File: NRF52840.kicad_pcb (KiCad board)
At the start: 2 copper layers, 31.2 x 11.3 mm, 26 parts, among them J1 Conn_01x04, J2 USB_A, U1 nRF52840, Y1 32M

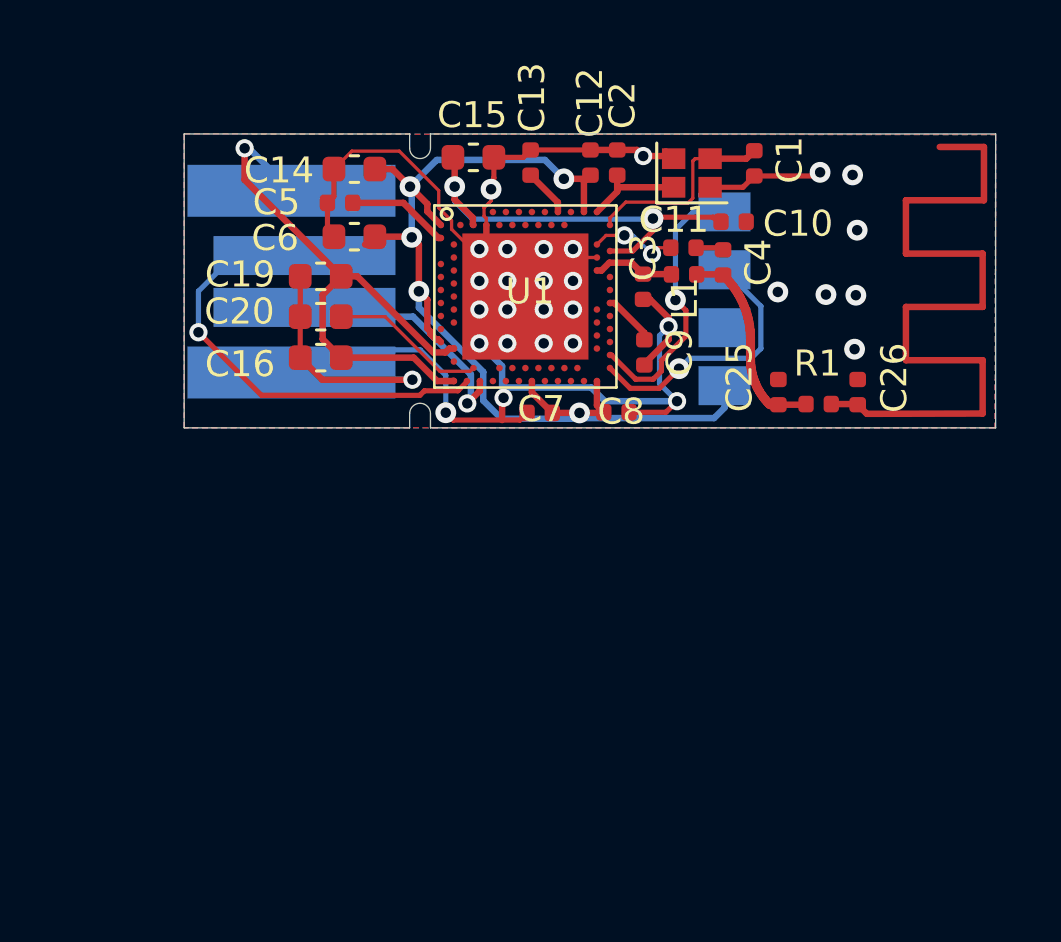
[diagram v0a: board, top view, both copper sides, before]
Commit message: ...
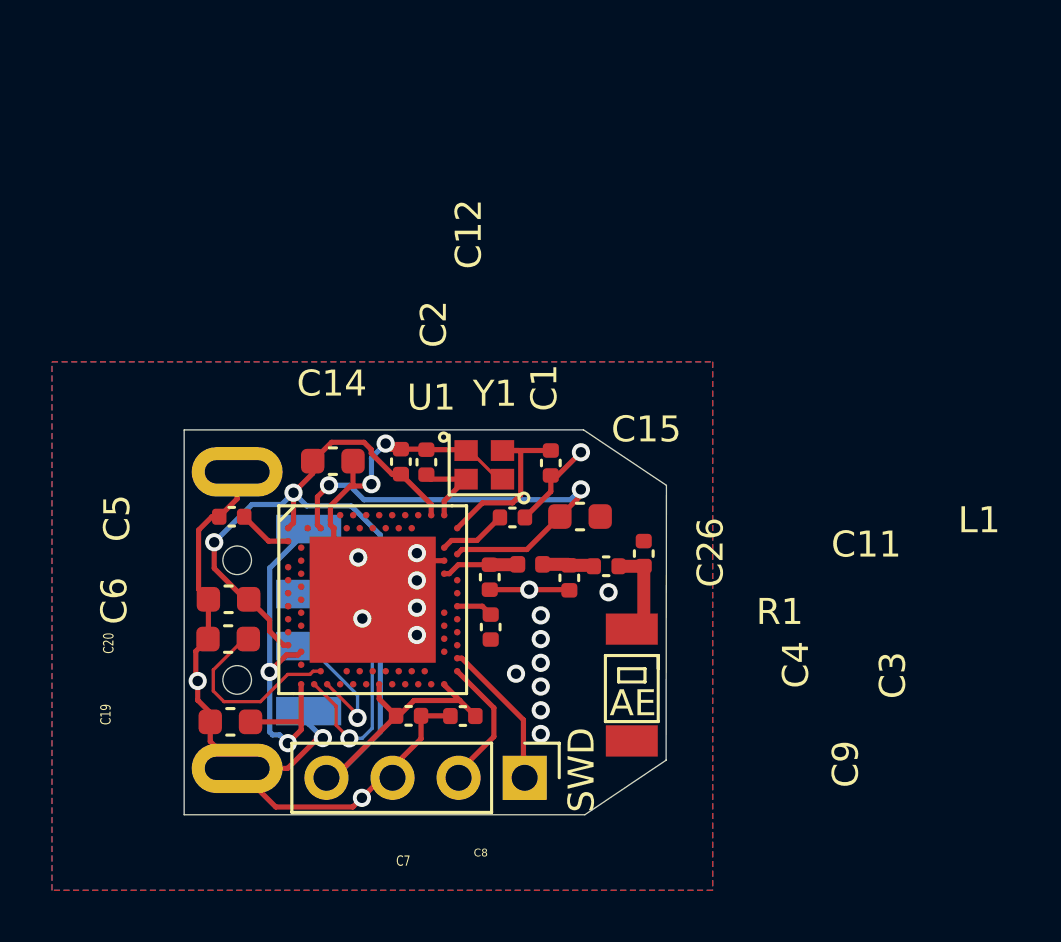
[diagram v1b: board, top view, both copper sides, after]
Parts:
- removed C10, C13, C25: NC, Capacitor_SMD:C_0402_1005Metric
- removed C16: 4.7uF, Capacitor_SMD:C_0603_1608Metric
- removed J1: Conn_01x04, zhangxiaofei:SWD
- added AE: Antenna, zhangxiaofei:2.4g_ANTENNA, F.Cu at (107.2, 141.8)
- added SWD: Conn_01x04, Connector_PinHeader_2.54mm:PinHeader_1x04_P2.54mm_Vertical, F.Cu at (103.1, 145.5)
- J2: footprint zhangxiaofei:USB_PCB -> Connector_USB:USB_A_CNCTech_1001-011-01101_Horizontal
- U1: footprint Package_DFN_QFN:Nordic_AQFN-73-1EP_7x7mm_P0.5mm -> zhangxiaofei:Nordic_AQFN-73-1EP_7x7mm_P0.5mm
- moved C19 17.5 mm to (91.8, 143.3)
- moved J2 15.9 mm to (85.2, 139.4), turned to 180 degrees
- moved C6 14.8 mm to (91.7, 138.6)
- moved C15 14.4 mm to (105.2, 135.4)
- moved C1 13.9 mm to (104.1, 133.3)
- moved Y1 13.8 mm to (101.6, 133.4)
- moved C2 13.7 mm to (99.3, 133.3)
- moved C12 13.6 mm to (98.4, 133.3)
- moved C4 13.5 mm to (104.8, 137.8), turned to 270 degrees
- moved C8 13.1 mm to (100.7, 143.1), turned to 180 degrees
- moved U1 13.1 mm to (97.3, 138.6)
- moved C20 12.9 mm to (91.7, 140.1)
- moved C5 12.8 mm to (91.9, 135.4)
- moved C7 12.7 mm to (98.7, 143.1), turned to 0 degrees
- moved C3 12.6 mm to (101.8, 137.7)
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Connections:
- U1 pad A10: Net-(U1-PadA10) -> (no net)
- U1 pad A12: Net-(U1-PadA12) -> (no net)
- U1 pad A14: Net-(U1-PadA14) -> (no net)
- U1 pad A16: Net-(U1-PadA16) -> (no net)
- U1 pad A18: Net-(C13-Pad2) -> (no net)
- U1 pad A20: Net-(U1-PadA20) -> (no net)
- U1 pad A8: Net-(U1-PadA8) -> (no net)
- U1 pad AB2: Net-(U1-PadAB2) -> (no net)
- U1 pad AC11: Net-(U1-PadAC11) -> (no net)
- U1 pad AC13: Net-(U1-PadAC13) -> (no net)
- U1 pad AC15: Net-(U1-PadAC15) -> (no net)
- U1 pad AC17: Net-(U1-PadAC17) -> (no net)
- U1 pad AC19: Net-(U1-PadAC19) -> (no net)
- U1 pad AC21: Net-(U1-PadAC21) -> (no net)
- U1 pad AC9: Net-(U1-PadAC9) -> (no net)
- U1 pad AD10: Net-(U1-PadAD10) -> (no net)
- U1 pad AD12: Net-(U1-PadAD12) -> (no net)
- U1 pad AD16: Net-(U1-PadAD16) -> (no net)
- U1 pad AD18: Net-(U1-PadAD18) -> (no net)
- U1 pad AD20: Net-(U1-PadAD20) -> (no net)
- U1 pad AD22: Net-(U1-PadAD22) -> (no net)
- U1 pad AD8: Net-(U1-PadAD8) -> (no net)
- U1 pad B11: Net-(U1-PadB11) -> (no net)
- U1 pad B13: Net-(U1-PadB13) -> (no net)
- U1 pad B15: Net-(U1-PadB15) -> (no net)
- U1 pad B17: Net-(U1-PadB17) -> (no net)
- U1 pad B19: Net-(U1-PadB19) -> (no net)
- U1 pad B3: Net-(U1-PadB3) -> (no net)
- U1 pad B9: Net-(U1-PadB9) -> (no net)
- U1 pad D2: Net-(U1-PadD2) -> (no net)
- U1 pad F2: Net-(U1-PadF2) -> (no net)
- U1 pad G1: Net-(U1-PadG1) -> (no net)
- U1 pad H2: Net-(U1-PadH2) -> (no net)
- U1 pad J1: Net-(U1-PadJ1) -> (no net)
- U1 pad J24: Net-(U1-PadJ24) -> (no net)
- U1 pad K2: Net-(U1-PadK2) -> (no net)
- U1 pad L1: Net-(U1-PadL1) -> (no net)
- U1 pad L24: Net-(U1-PadL24) -> (no net)
- U1 pad M2: Net-(U1-PadM2) -> (no net)
- U1 pad N1: Net-(U1-PadN1) -> (no net)
- U1 pad P2: Net-(U1-PadP2) -> (no net)
- U1 pad P23: Net-(U1-PadP23) -> (no net)
- U1 pad R1: Net-(U1-PadR1) -> (no net)
- U1 pad R24: Net-(U1-PadR24) -> (no net)
- U1 pad T2: Net-(U1-PadT2) -> (no net)
- U1 pad T23: Net-(U1-PadT23) -> (no net)
- U1 pad U1: Net-(U1-PadU1) -> (no net)
- U1 pad U24: Net-(U1-PadU24) -> (no net)
- U1 pad V23: Net-(U1-PadV23) -> (no net)
- U1 pad W24: Net-(U1-PadW24) -> (no net)
- U1 pad Y23: Net-(U1-PadY23) -> (no net)
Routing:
- net GND: track 79.6 -> 53.2 mm, vias 30 -> 21
- net Net-(AE1-Pad1): track 29.8 -> 3.58 mm
- net +5V: track 35.3 -> 15.6 mm, vias 1 -> 2
- net D-: track 17.8 -> 9.96 mm
- net Net-(C4-Pad1): track 7.90 -> 1.99 mm
- net SWDIO: track 10.4 -> 5.08 mm, vias 1 -> 0
- net SWDCLK: track 10.7 -> 5.58 mm, vias 1 -> 0
- net Net-(C5-Pad1): track 3.95 -> 2.08 mm
- net Net-(C13-Pad2): track 1.85 -> 0.00 mm
- net Net-(C20-Pad1): track 6.00 -> 7.43 mm
- net Net-(C15-Pad1): track 16.5 -> 17.9 mm
- net D+: track 6.31 -> 5.31 mm
- net Net-(C11-Pad2): track 3.38 -> 2.62 mm, vias 2 -> 0
- net Net-(C9-Pad1): track 2.07 -> 1.42 mm
- net Net-(C1-Pad2): track 7.76 -> 7.13 mm
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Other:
- board size 31.2 x 11.3 mm -> 18.5 x 14.8 mm
- board text added: "3.3"
- board text added: "CLK"
- board text added: "IO"
- board text removed: "3V3"
- board text removed: "5"
- board text removed: "D+"
- board text removed: "D-"
- board text removed: "SWDCLK"
- board text removed: "SWDIO"
